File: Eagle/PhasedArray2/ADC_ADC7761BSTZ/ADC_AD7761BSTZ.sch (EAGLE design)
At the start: 42 parts, among them U1 AD7761BSTZ, Y1 HCM4932768000ABJT

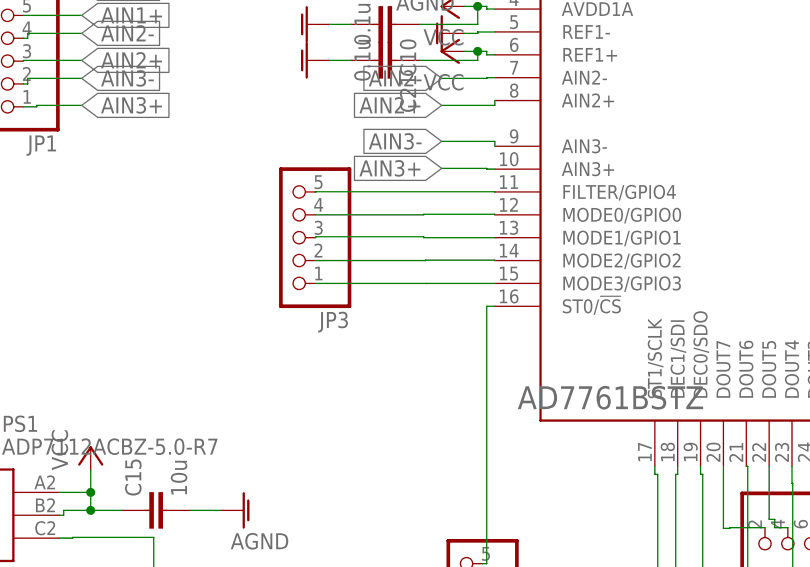
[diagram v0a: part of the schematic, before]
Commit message: Add files via upload
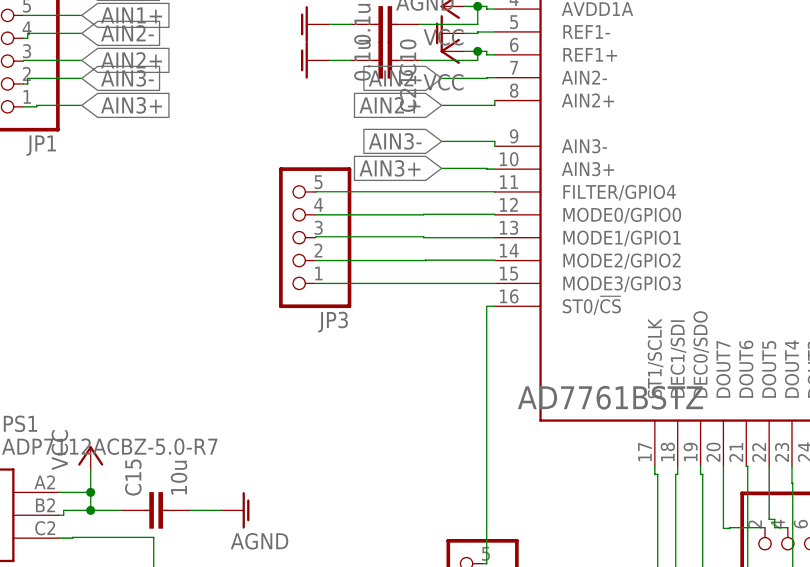
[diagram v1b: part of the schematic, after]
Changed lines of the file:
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@@
 <segment>
 <pinref part="U1" gate="G$1" pin="MODE3/GPIO3"/>
-<wire x1="-45.7" y1="-17.8" x2="-45.7" y2="-17.78" width="0.1524" layer="91"/>
-<wire x1="-45.7" y1="-17.78" x2="-38.1" y2="-17.78" width="0.1524" layer="91"/>
 <pinref part="JP3" gate="A" pin="1"/>
-<wire x1="-45.7" y1="-17.78" x2="-58.06" y2="-17.78" width="0.1524" layer="91"/>
+<wire x1="-38.1" y1="-17.78" x2="-58.06" y2="-17.78" width="0.1524" layer="91"/>
 </segment>
 </net>
